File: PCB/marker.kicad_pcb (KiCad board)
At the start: 4 copper layers, 39.5 x 94 mm, 57 parts, among them J1 2216100001, U1 W25Q128JVS, U2 RP2040, U3 DWM1001

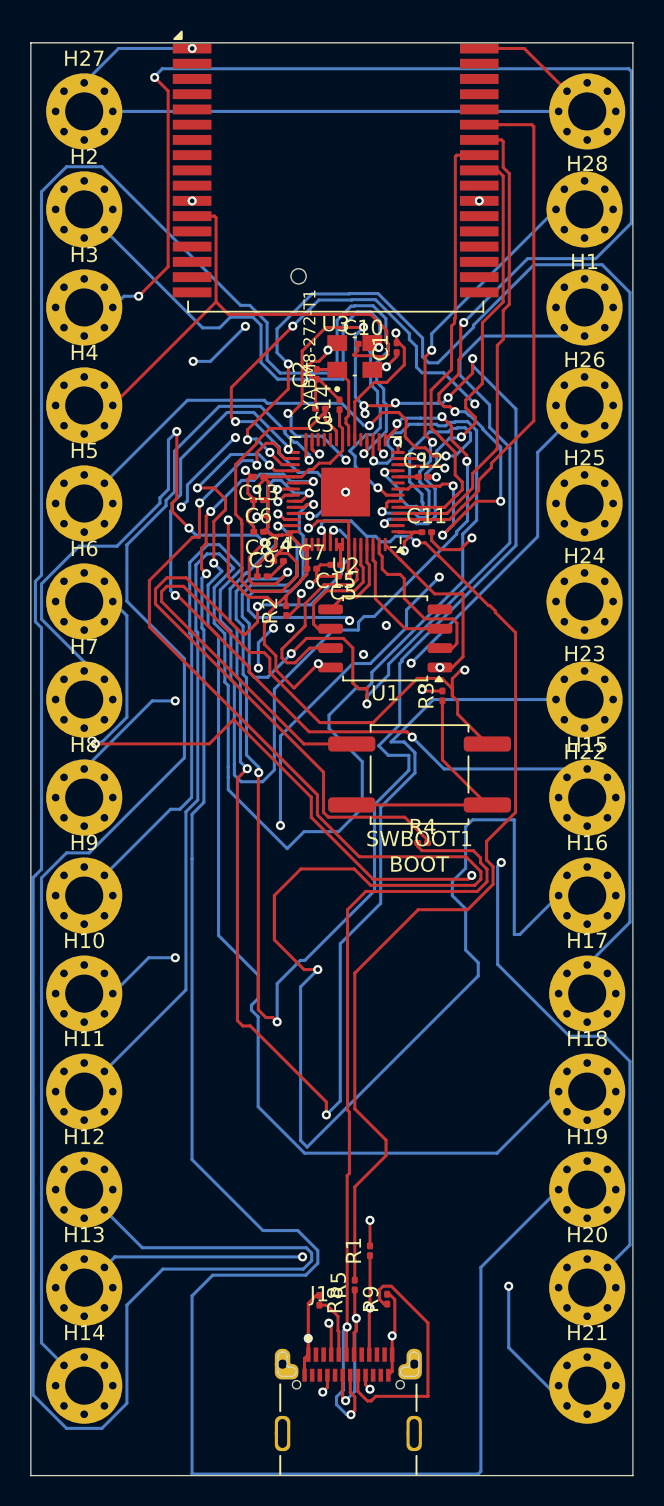
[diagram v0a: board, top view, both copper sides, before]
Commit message: fixing things
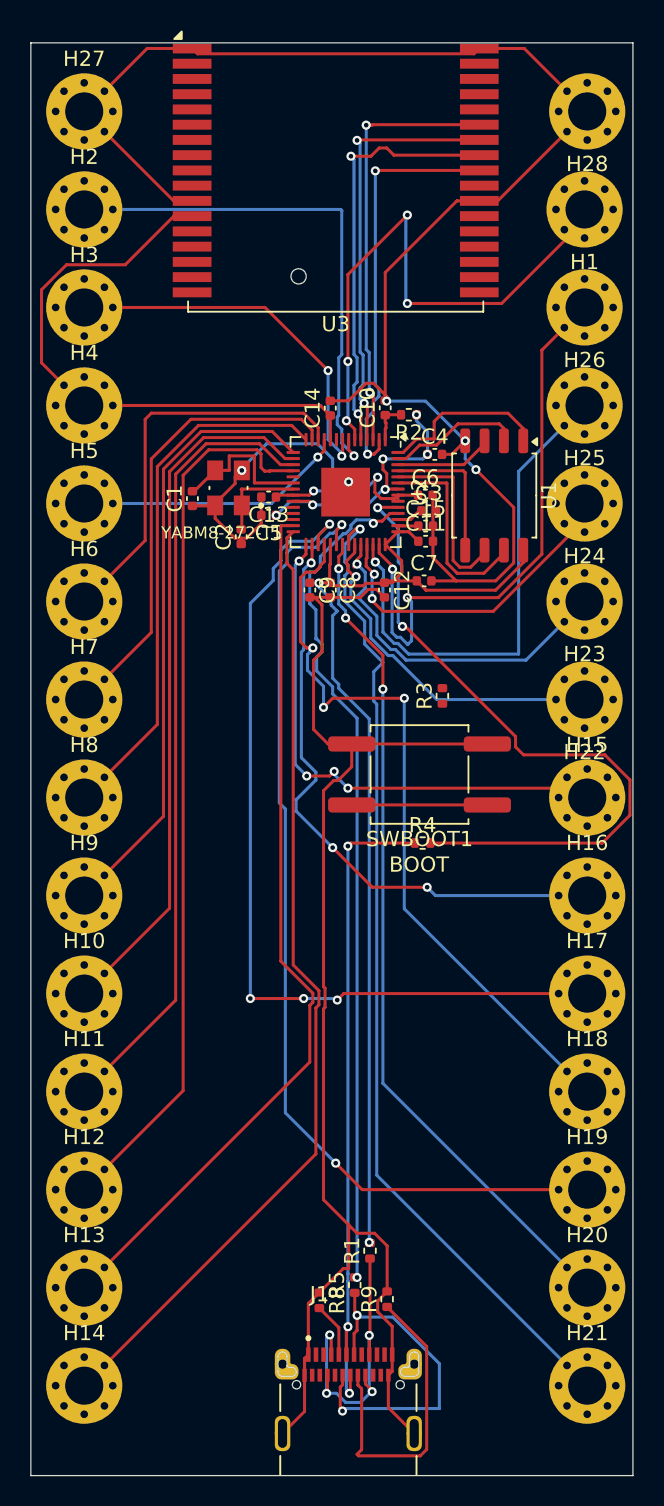
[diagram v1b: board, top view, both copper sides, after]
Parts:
- C1, C10, C11, C12, C13, C14, C15, C2, C3, C4, C5, C6, C7, C8, C9: footprint Capacitor_SMD:C_0201_0603Metric -> Capacitor_SMD:C_0402_1005Metric
- R1, R2, R3, R4, R5, R8, R9: footprint Resistor_SMD:R_0201_0603Metric -> Resistor_SMD:R_0402_1005Metric
- moved C1 16.7 mm to (105.1, 70.9)
- moved R2 15.2 mm to (119.3, 65.4), turned to 180 degrees
- moved C4 12.4 mm to (121.0, 68.0)
- moved YABM8-272-T1 12.0 mm to (107.5, 70.2), turned to 180 degrees
- moved U1 11.8 mm to (124.9, 70.7), turned to -90 degrees
- moved C2 11.7 mm to (108.3, 73.4)
- moved C6 11.0 mm to (120.4, 70.7), turned to 0 degrees
- moved C3 9.76 mm to (120.6, 71.7), turned to 0 degrees
- moved C12 7.85 mm to (117.7, 76.9), turned to -90 degrees
- moved C7 7.41 mm to (120.3, 76.3)
- moved C15 6.43 mm to (120.4, 72.7), turned to 0 degrees
- moved C5 6.33 mm to (110.1, 72.0)
- moved C8 6.07 mm to (114.1, 76.9), turned to -90 degrees
- moved C10 4.44 mm to (117.7, 64.9), turned to 90 degrees
- moved C9 3.25 mm to (112.8, 76.9), turned to -90 degrees
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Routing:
- net Net-(U2-GPIO10): track 168.2 -> 30.2 mm, vias 15 -> 0
- net GND: track 344.4 -> 219.9 mm, vias 13 -> 5
- net Net-(U2-GPIO15): track 169.8 -> 58.6 mm, vias 1 -> 0
- net Net-(U2-GPIO19): track 128.1 -> 40.1 mm
- net Net-(U2-GPIO6): track 102.3 -> 24.8 mm, vias 7 -> 2
- net Net-(U2-GPIO25): track 92.6 -> 23.1 mm, vias 3 -> 1
- net Net-(U2-GPIO22): track 126.3 -> 64.8 mm, vias 3 -> 2
- net Net-(U2-GPIO24): track 125.1 -> 65.4 mm, vias 2 -> 1
- net Net-(U2-GPIO9): track 83.2 -> 26.3 mm, vias 4 -> 0
- net Net-(U2-GPIO14): track 108.8 -> 52.1 mm, vias 1 -> 0
- net Net-(U2-GPIO12): track 82.4 -> 40.2 mm, vias 3 -> 0
- net +3.3V: track 163.7 -> 124.3 mm, vias 7 -> 4
- net Net-(U2-GPIO23): track 90.0 -> 55.6 mm, vias 6 -> 3
- net Net-(U2-GPIO20): track 92.1 -> 58.1 mm, vias 3 -> 4
- net Net-(U2-GPIO21): track 79.2 -> 49.3 mm
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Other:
- copper layers 4 -> 2
